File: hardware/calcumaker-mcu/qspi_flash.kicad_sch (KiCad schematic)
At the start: 3 parts, among them U7 W25Q32JVSSIQ

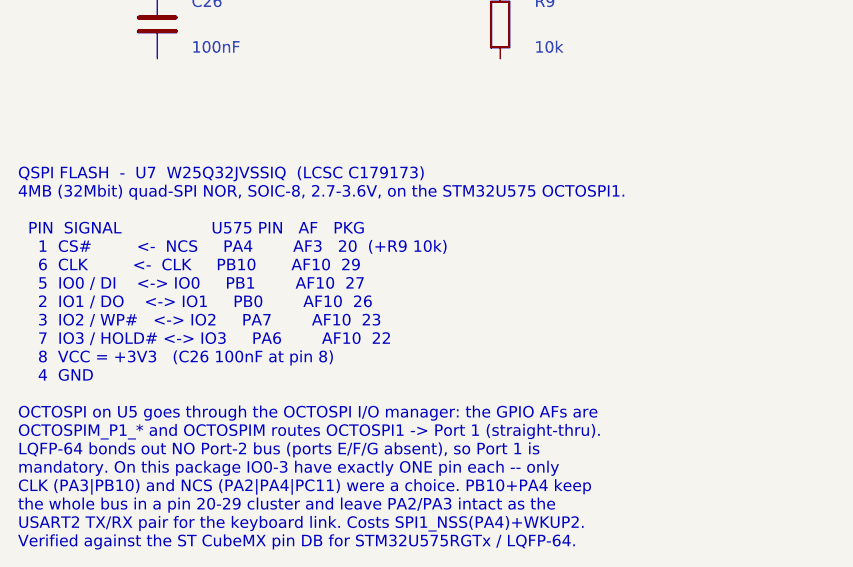
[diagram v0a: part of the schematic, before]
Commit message: Checkpoint
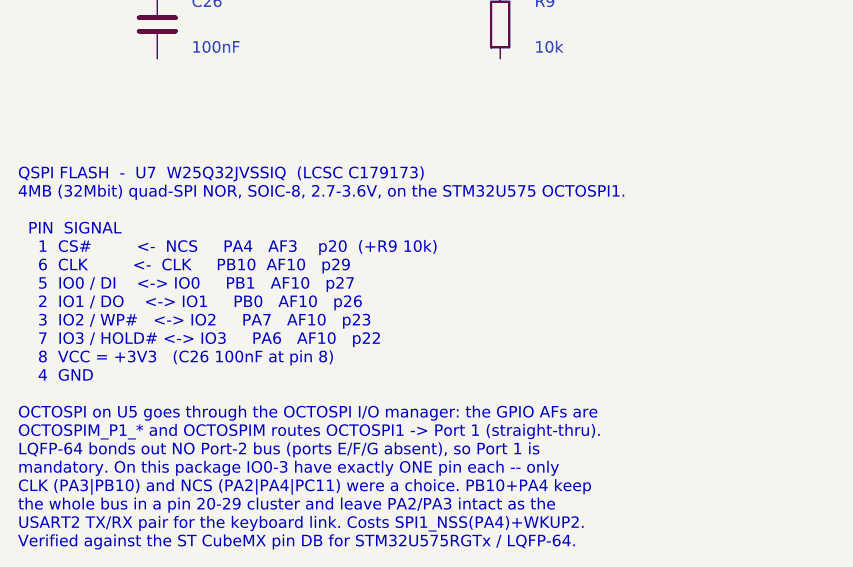
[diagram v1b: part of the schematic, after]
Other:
- note added: "QSPI FLASH - U7 W25Q32JVSSIQ (LCSC C179173) 4MB (32Mbit) quad-SPI NOR, SOIC-8, 2.7-3.6V, on the STM32U575 OCTOSPI1. PIN SIGNAL 1 CS# <- NCS PA4 AF3 p20 (+R9 10k) 6 CLK <- CLK PB10 AF10 p29 5 IO0 / DI <-> IO0 PB1 AF10 p27 2 IO1 / DO <-> IO1 PB0 AF10 p26 3 IO2 / WP# <-> IO2 PA7 AF10 p23 7 IO3 / HOLD# <-> IO3 PA6 AF10 p22 8 VCC = +3V3 (C26 100nF at pin 8) 4 GND OCTOSPI on U5 goes through the OCTOSPI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"
- note removed: "QSPI FLASH - U7 W25Q32JVSSIQ (LCSC C179173) 4MB (32Mbit) quad-SPI NOR, SOIC-8, 2.7-3.6V, on the STM32U575 OCTOSPI1. PIN SIGNAL U575 PIN AF PKG 1 CS# <- NCS PA4 AF3 20 (+R9 10k) 6 CLK <- CLK PB10 AF10 29 5 IO0 / DI <-> IO0 PB1 AF10 27 2 IO1 / DO <-> IO1 PB0 AF10 26 3 IO2 / WP# <-> IO2 PA7 AF10 23 7 IO3 / HOLD# <-> IO3 PA6 AF10 22 8 VCC = +3V3 (C26 100nF at pin 8) 4 GND OCTOSPI on U5 goes through t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"
